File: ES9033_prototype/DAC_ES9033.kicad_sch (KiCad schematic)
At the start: 31 parts, among them U201 ES9033, X201 ECS-2520MV-xxx-xx

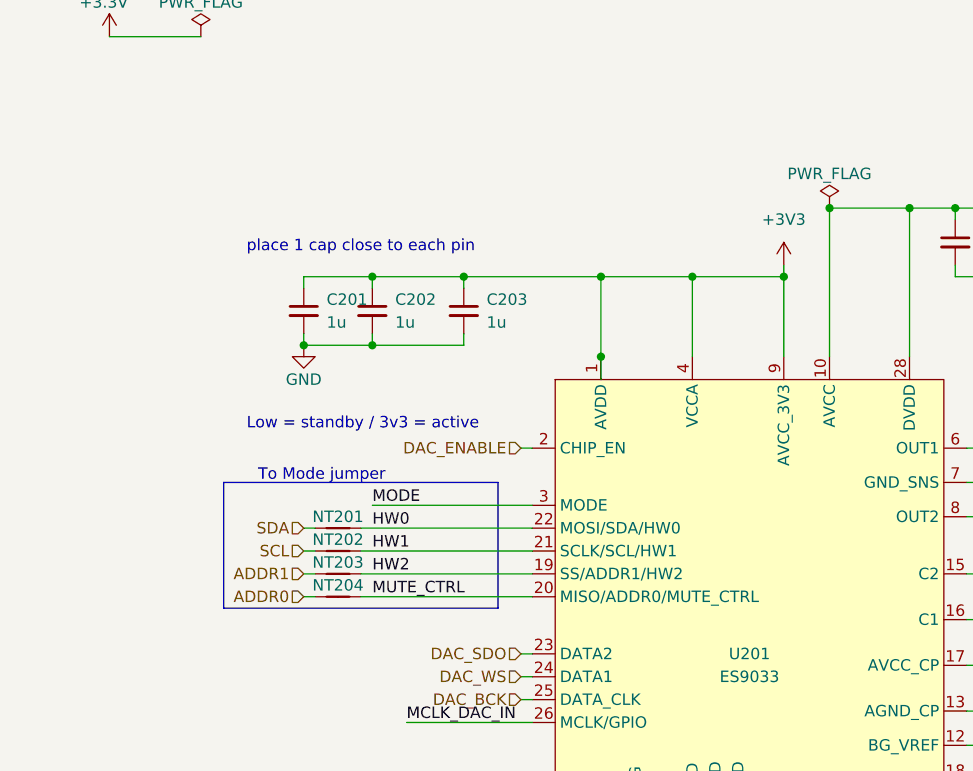
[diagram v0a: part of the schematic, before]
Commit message: stuff
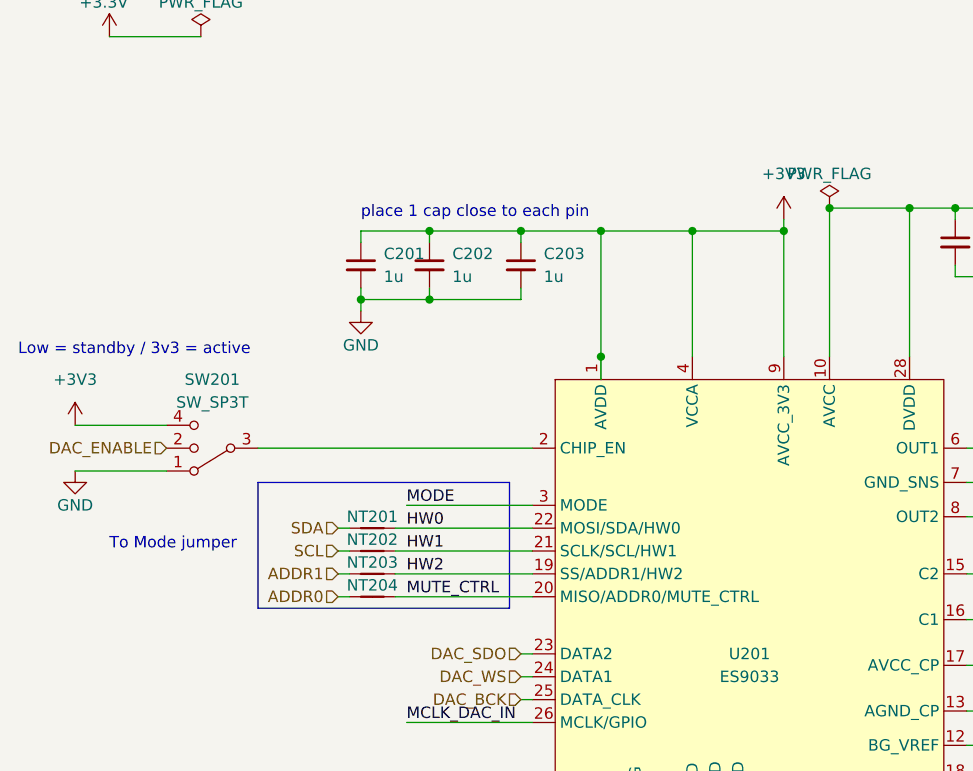
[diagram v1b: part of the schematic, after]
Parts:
- added SW201: SW_SP3T, Button_Switch_SMD:SW_SP3T_PCM13, symbol Switch:SW_SP3T
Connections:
- net +3V3: now also SW201.4
- net DAC_ENABLE: now also SW201.2; no longer U201.2 (CHIP_EN)
- net GND: now also SW201.1
- new net: SW201.3, U201.2 (CHIP_EN)
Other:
- moved on the sheet: C201, C202, C203, NT201, NT202, NT203, NT204
